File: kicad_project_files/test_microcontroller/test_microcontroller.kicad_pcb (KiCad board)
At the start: 2 copper layers, 60 x 84 mm, 41 parts, among them J1 USB_C_Receptacle_USB2.0, SW1 SW_Push, SW2 SW_Push, SW3 SW_Push, SW4 SW_Push, SW5 SW_Push, SW6 SW_Push, SW7 SW_Push, SW8 SW_Push, SW9 SW_Push, U1 ATmega8U2-A, Y1 16mhz

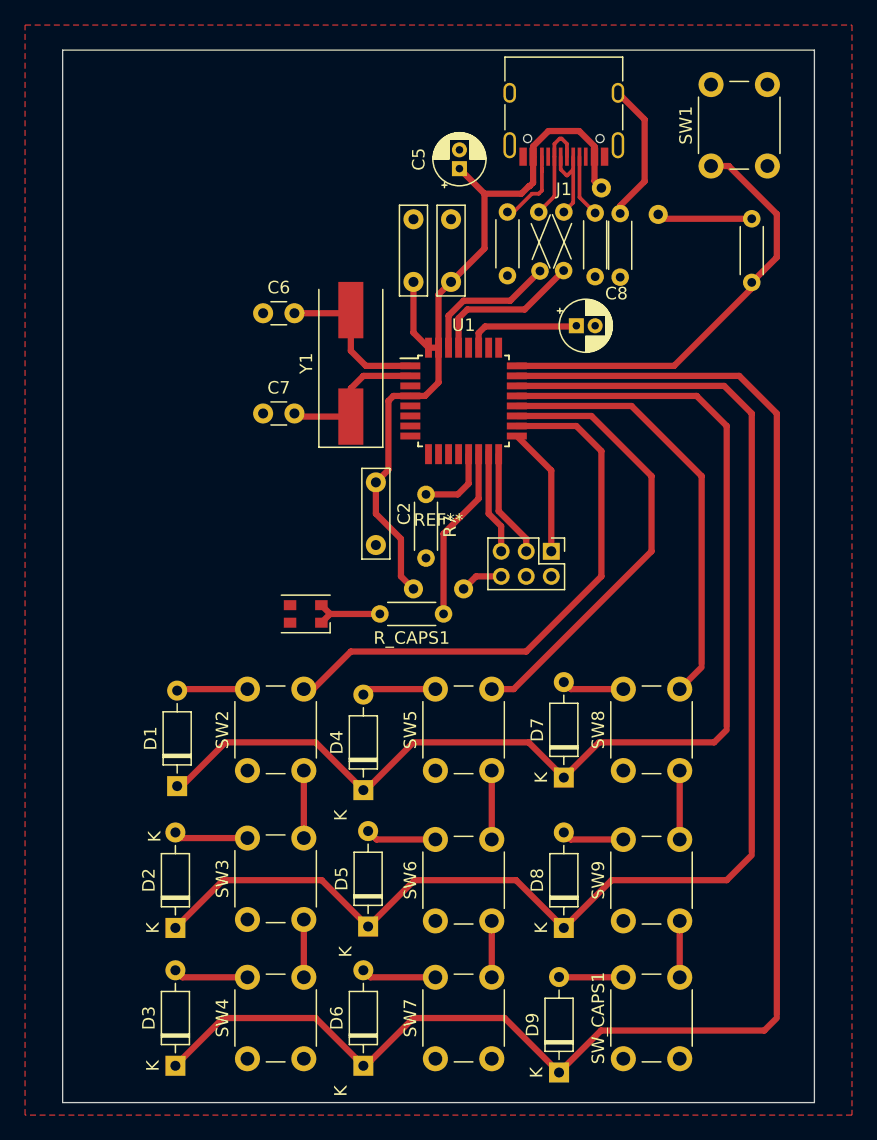
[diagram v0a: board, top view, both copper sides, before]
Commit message: update pcb
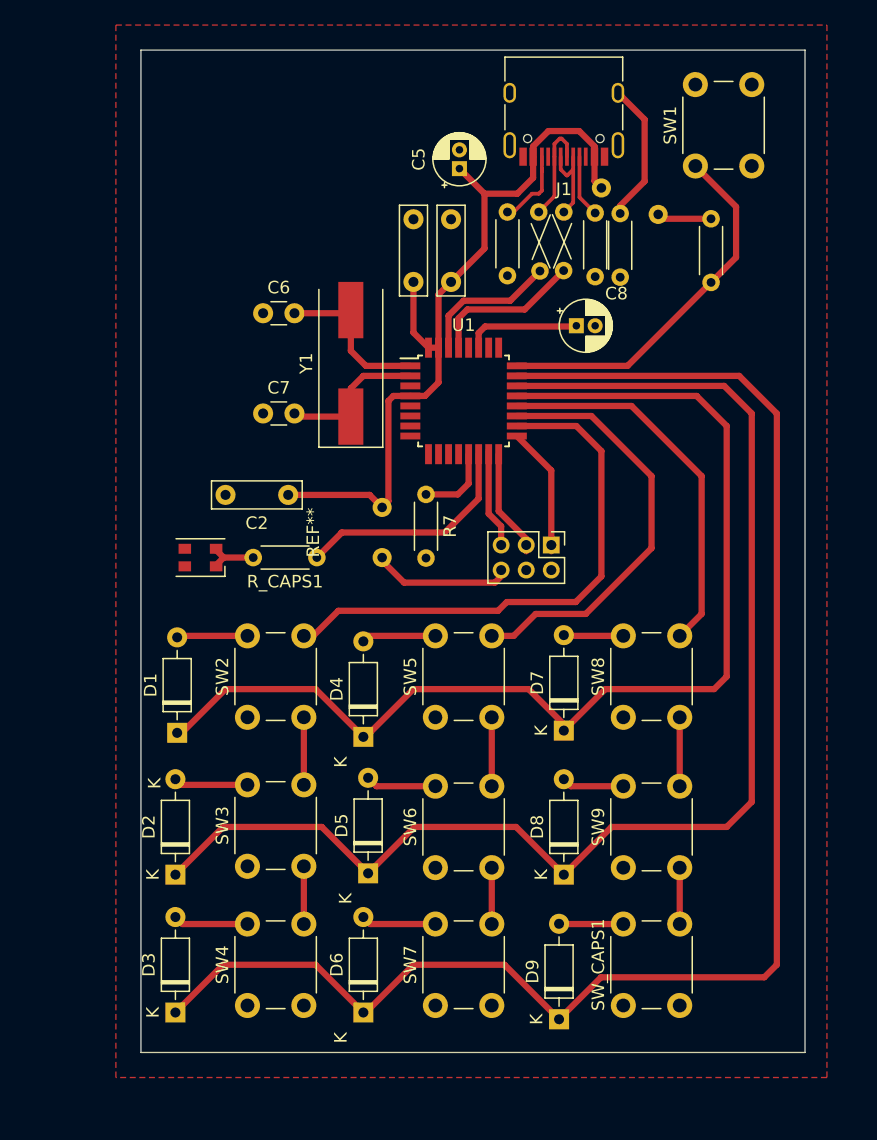
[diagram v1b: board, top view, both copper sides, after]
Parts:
- moved R_CAPS1 11.1 mm to (49.3, 60.5)
- moved D_CAPS1 9.53 mm to (40.0, 60.5)
- moved REF** 9.51 mm to (49.5, 58.5), turned to 90 degrees
- moved C2 7.07 mm to (47.0, 55.5), turned to 180 degrees
- moved D1 4.25 mm to (38.1, 74.5)
- moved D2 4.25 mm to (38.0, 85.8)
- moved D3 4.25 mm to (38.0, 96.8)
- moved D4 4.25 mm to (53.0, 74.8)
- moved D5 4.25 mm to (53.4, 85.7)
- moved D6 4.25 mm to (53.0, 96.8)
- moved D8 4.25 mm to (69.0, 85.8)
- moved D9 4.25 mm to (68.6, 97.3)
- moved SW2 4.25 mm to (43.8, 73.2)
- moved SW3 4.25 mm to (43.8, 85.1)
- moved SW4 4.25 mm to (43.8, 96.2)
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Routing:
- net RESET: track 34.9 -> 29.7 mm
- net CAPS: track 13.9 -> 18.4 mm
- net ROW3: track 126.3 -> 122.3 mm
- net ROW2: track 109.3 -> 105.3 mm
- net COL3: track 44.5 -> 40.5 mm
- net VCC: track 74.9 -> 78.4 mm
- net ROW1: track 92.9 -> 89.7 mm
- net COL2: track 46.0 -> 44.1 mm
- net COL1: track 55.1 -> 53.3 mm
- net Net-(R_CAPS1-Pad2): track 5.95 -> 4.19 mm
- net SCLK: track 8.41 -> 7.91 mm
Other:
- board size 60 x 84 mm -> 53 x 80 mm
